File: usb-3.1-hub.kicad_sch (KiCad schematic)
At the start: 45 parts, among them J1 Conn_01x09, J2 Conn_01x05, J3 Conn_01x09, J4 Conn_01x09, J5 Conn_01x09, J6 Conn_01x09, Q4 NPN, Q5 NPN, Q6 NPN, U1 GL3510, Y1 Crystal_GND24

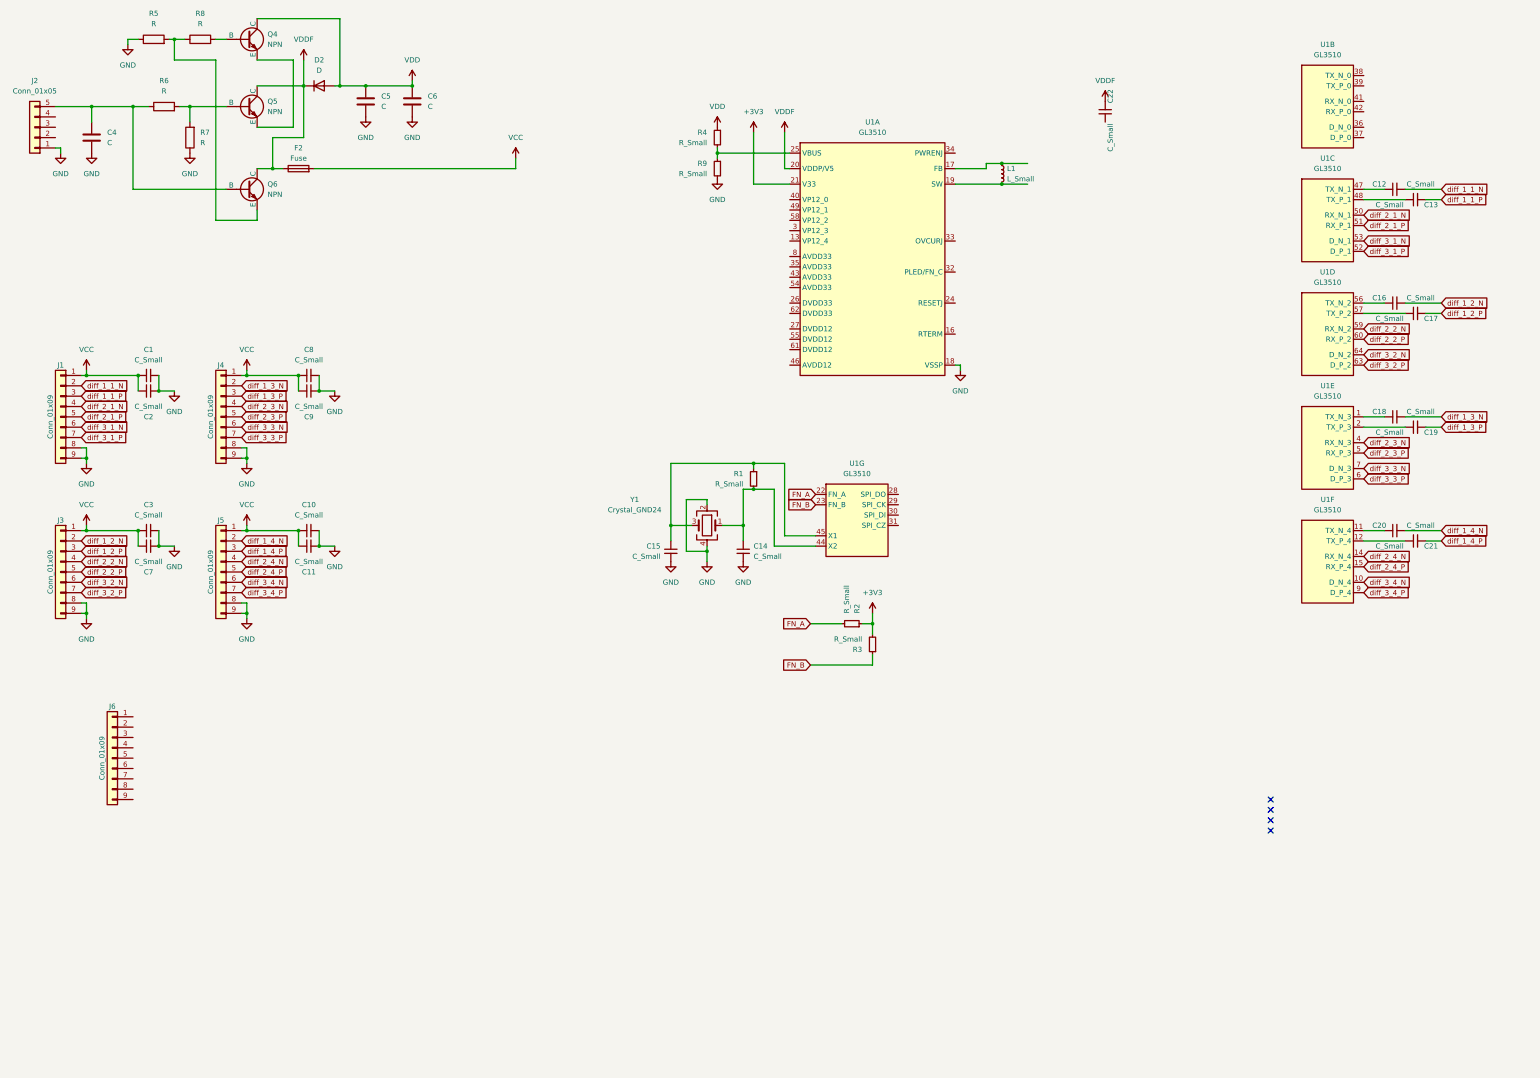
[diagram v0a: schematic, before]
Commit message: Prepared schematic
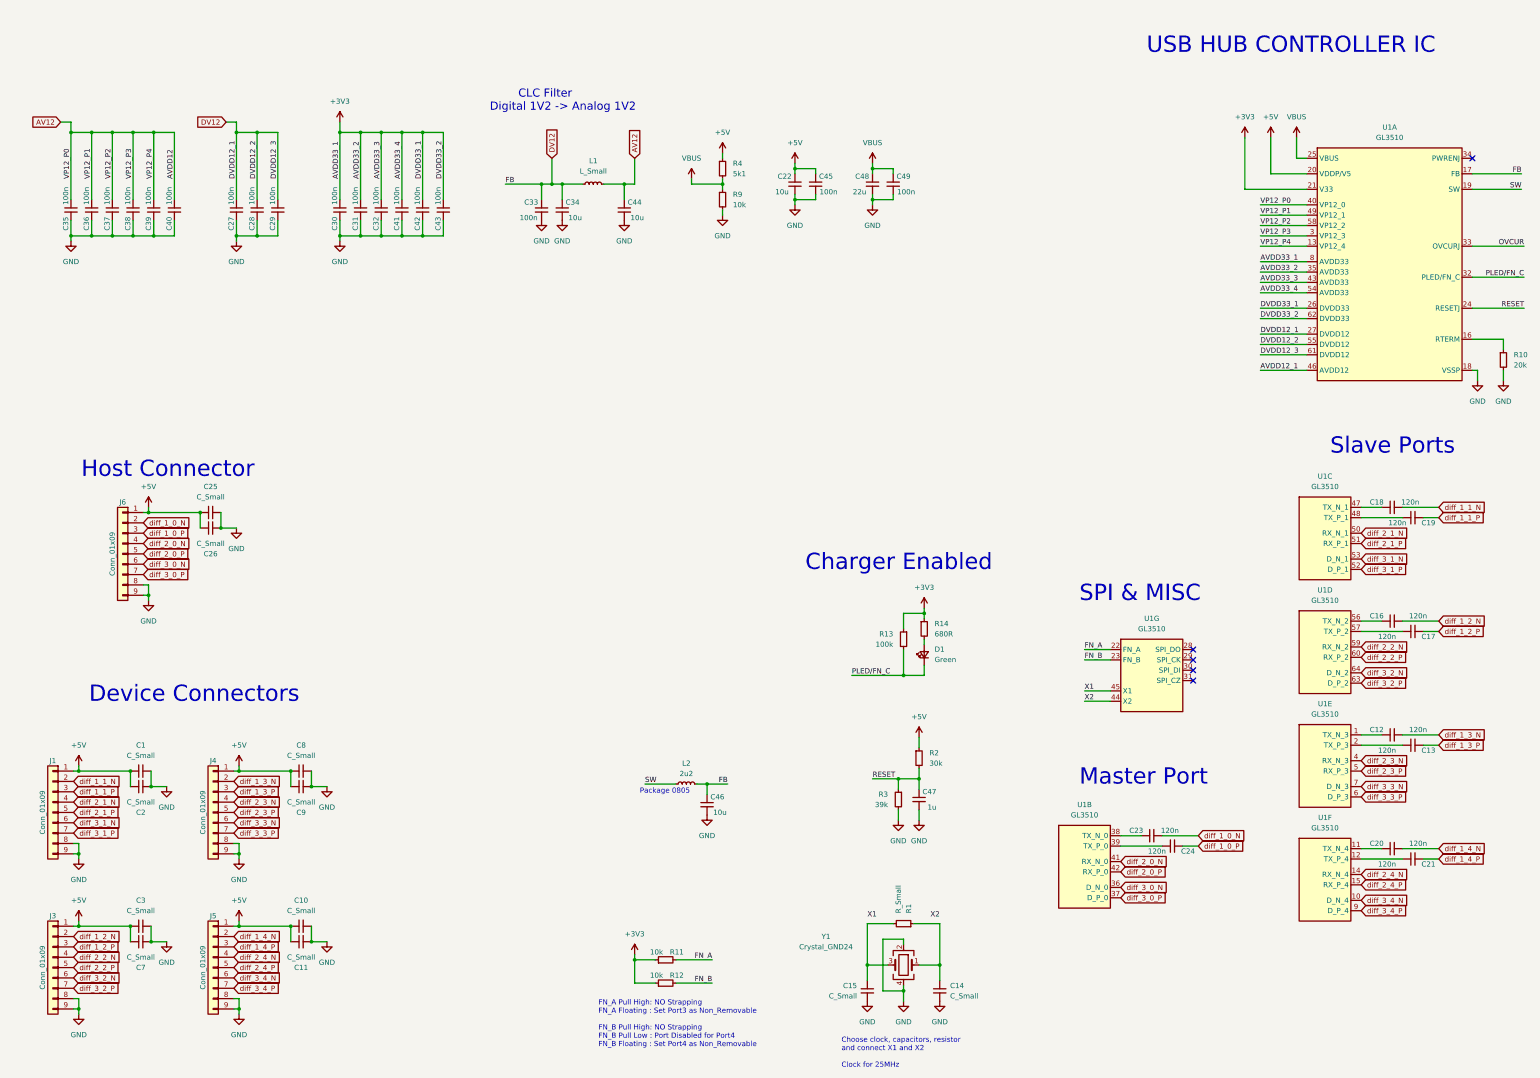
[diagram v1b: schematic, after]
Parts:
- removed C4, C5, C6: C, symbol Device:C
- removed D2: D, symbol Device:D
- removed F2: Fuse, symbol Device:Fuse
- removed J2: Conn_01x05, symbol Connector_Generic:Conn_01x05
- removed Q4, Q5, Q6: NPN, symbol Simulation_SPICE:NPN
- removed R5, R6, R7, R8: R, symbol Device:R
- added C23, C24: 120n, symbol Device:C_Small
- added C25, C26: C_Small, symbol Device:C_Small
- added C27, C28, C29, C30, C31, C32, C33, C35, C36, C37, C38, C39, C40, C41, C42, C43, C45, C49: 100n, symbol Device:C_Small
- added C34, C44, C46: 10u, symbol Device:C_Small
- added C47: 1u, symbol Device:C_Small
- added C48: 22u, symbol Device:C_Small
- added D1: Green, symbol Device:LED_Small
- added L2: 2u2, symbol Device:L_Small
- added R10: 20k, symbol Device:R_Small
- added R11, R12: 10k, symbol Device:R_Small
- added R13: 100k, symbol Device:R_Small
- added R14: 680R, symbol Device:R_Small
- C12, C13, C16, C17, C18, C19, C20, C21: value C_Small -> 120n
- C22: value C_Small -> 10u
- R2: value R_Small -> 30k
- R3: value R_Small -> 39k
- R4: value R_Small -> 5k1
- R9: value R_Small -> 10k
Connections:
- net VCC is gone; now on net +5V: C1.1, C10.1, C11.1, C2.1, C3.1, C7.1, C8.1, C9.1, J1.1 (Pin_1), J3.1 (Pin_1), J4.1 (Pin_1), J5.1 (Pin_1)
- net VDD is gone; now on net +5V: R4.1
- net VDDF is gone; now on net +5V: C22.1, U1.20 (VDDP/V5)
- net +3V3: now also U1.26 (DVDD33), U1.35 (AVDD33), U1.43 (AVDD33), U1.54 (AVDD33), U1.62 (DVDD33), U1.8 (AVDD33), C30.1, C31.1, C32.1, C41.1, C42.1, C43.1, R11.1, R12.1, R13.1, R14.1; no longer R2.1, R3.2
- net FN_A: now also R11.2; no longer R2.2
- net FN_B: now also R12.2; no longer R3.1
- net GND: now also C22.2, J6.8 (Pin_8), J6.9 (Pin_9), R3.2, C25.2, C26.2, C27.2, C28.2, C29.2, C30.2, C31.2, C32.2, C33.2, C34.2, C35.2, C36.2, C37.2, C38.2, C39.2, C40.2, C41.2, C42.2, C43.2, C44.2, C45.2, C46.2, C47.2, C48.2, C49.2, R10.2
- net diff_1_1_N: now also C18.2; no longer C12.2
- net diff_1_1_P: now also C19.2; no longer C13.2
- net diff_1_3_N: now also C12.2; no longer C18.2
- net diff_1_3_P: now also C13.2; no longer C19.2
- net at C13.1: now also U1.2 (TX_P_3); no longer U1.48 (TX_P_1)
- net diff_3_0_N: now reaches U1.36 (D_N_0)
- net diff_3_0_N: now also J6.6 (Pin_6)
- net diff_3_0_P: now reaches U1.37 (D_P_0)
- net diff_3_0_P: now also J6.7 (Pin_7)
- net at U1.38 (TX_N_0): now also C23.1
- net at U1.39 (TX_P_0): now also C24.1
- net diff_2_0_N: now reaches U1.41 (RX_N_0)
- net diff_2_0_N: now also J6.4 (Pin_4)
- net diff_2_0_P: now reaches U1.42 (RX_P_0)
- net diff_2_0_P: now also J6.5 (Pin_5)
- net VBUS: now reaches R4.2, R9.1, U1.25 (VBUS)
- net VBUS: now also C48.1, C49.1
- net DV12: now reaches L1.1, U1.17 (FB)
- net DV12: now also U1.27 (DVDD12), U1.55 (DVDD12), U1.61 (DVDD12), C27.1, C28.1, C29.1, C33.1, C34.1, C46.1, L2.2
- net AV12: now reaches L1.2
- net AV12: now also U1.13 (VP12_4), U1.3 (VP12_3), U1.40 (VP12_0), U1.49 (VP12_1), U1.58 (VP12_2), C35.1, C36.1, C37.1, C38.1, C39.1, C40.1, C44.1; no longer U1.19 (SW)
- net at C19.1: now also U1.48 (TX_P_1); no longer U1.2 (TX_P_3)
- net at C18.1: now also U1.47 (TX_N_1); no longer U1.1 (TX_N_3)
- net at C14.1, Y1.1: now also R1.1; no longer R1.2, U1.44 (X2)
- net at C15.1, Y1.3: now also R1.2; no longer R1.1, U1.45 (X1)
- net +5V: now reaches J6.1 (Pin_1)
- net +5V: now also R2.1, C25.1, C26.1, C45.1
- net diff_1_0_N: now reaches J6.2 (Pin_2)
- net diff_1_0_N: now also C23.2
- net diff_1_0_P: now reaches J6.3 (Pin_3)
- net diff_1_0_P: now also C24.2
- net at U1.16 (RTERM): now also R10.1
- net RESET: now reaches U1.24 (RESETJ)
- net RESET: now also R2.2, R3.1, C47.1
- net PLED/FN_C: now reaches U1.32 (PLED/FN_C)
- net PLED/FN_C: now also D1.1 (K), R13.2
- net OVCUR: now reaches U1.33 (OVCURJ)
- net AVDD12_1: now reaches U1.46 (AVDD12)
- net at C12.1: now also U1.1 (TX_N_3); no longer U1.47 (TX_N_1)
- new net: D1.2 (A), R14.2
- new net SW: L2.1, U1.19 (SW)
- new net X1: U1.45 (X1)
- new net X2: U1.44 (X2)
- no-connect marks 4 -> 5
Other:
- note added: "CLC Filter Digital 1V2 -> Analog 1V2"
- note added: "Charger Enabled"
- note added: "Choose clock, capacitors, resistor and connect X1 and X2 Clock for 25MHz"
- note added: "Device Connectors"
- note added: "FN_A Pull High: NO Strapping FN_A Floating : Set Port3 as Non_Removable FN_B Pull High: NO Strapping FN_B Pull Low : Port Disabled for Port4 FN_B Floating : Set Port4 as Non_Removable"
- note added: "Host Connector"
- note added: "Master Port"
- note added: "Package 0805"
- note added: "SPI & MISC"
- note added: "Slave Ports"
- note added: "USB HUB CONTROLLER IC"
- moved on the sheet: C1, C10, C11, C14, C15, C2, C20, C21, C3, C7, C8, C9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
